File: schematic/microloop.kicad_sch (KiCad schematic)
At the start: 28 parts, among them J1 AudioJack3, J2 AudioJack3, SW1 RotaryEncoder_Switch, SW2 RotaryEncoder_Switch, SW3 RotaryEncoder_Switch, SW4 RotaryEncoder_Switch, SW5 SW_Push, SW6 SW_Push, SW7 SW_Push, SW8 SW_Push, U1 Teensy4.1, U2 Teensy4.0_AudioShield_REVD, U3 Adafruit MIDI Featherwing, U4 Adafruit NeoKey 1x4, U5 MCP23017_SO, U6 128×64 OLED

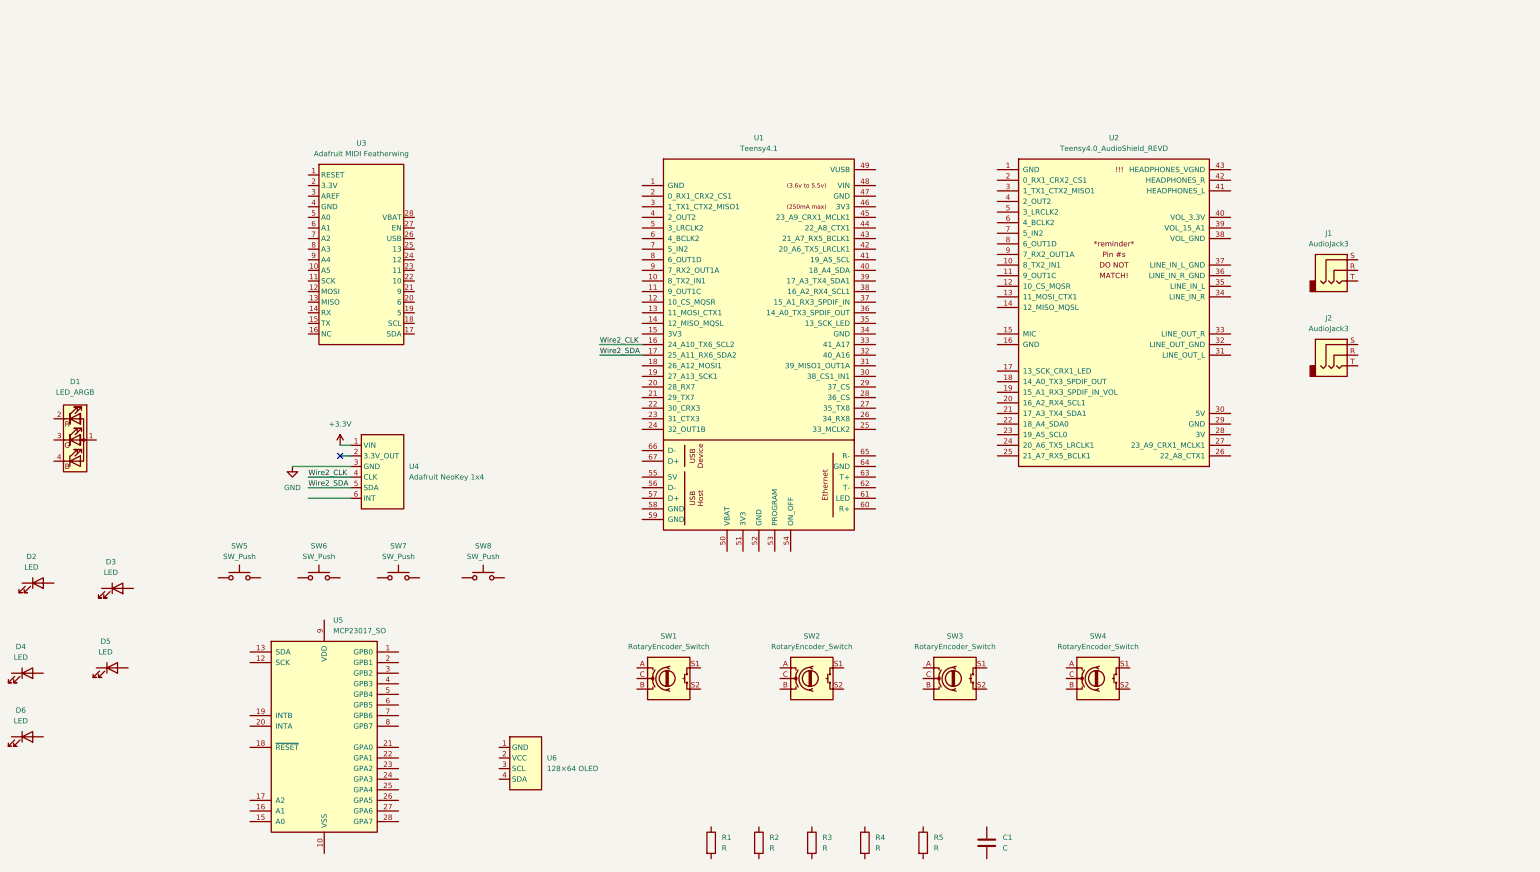
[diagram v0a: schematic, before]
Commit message: updated schematic
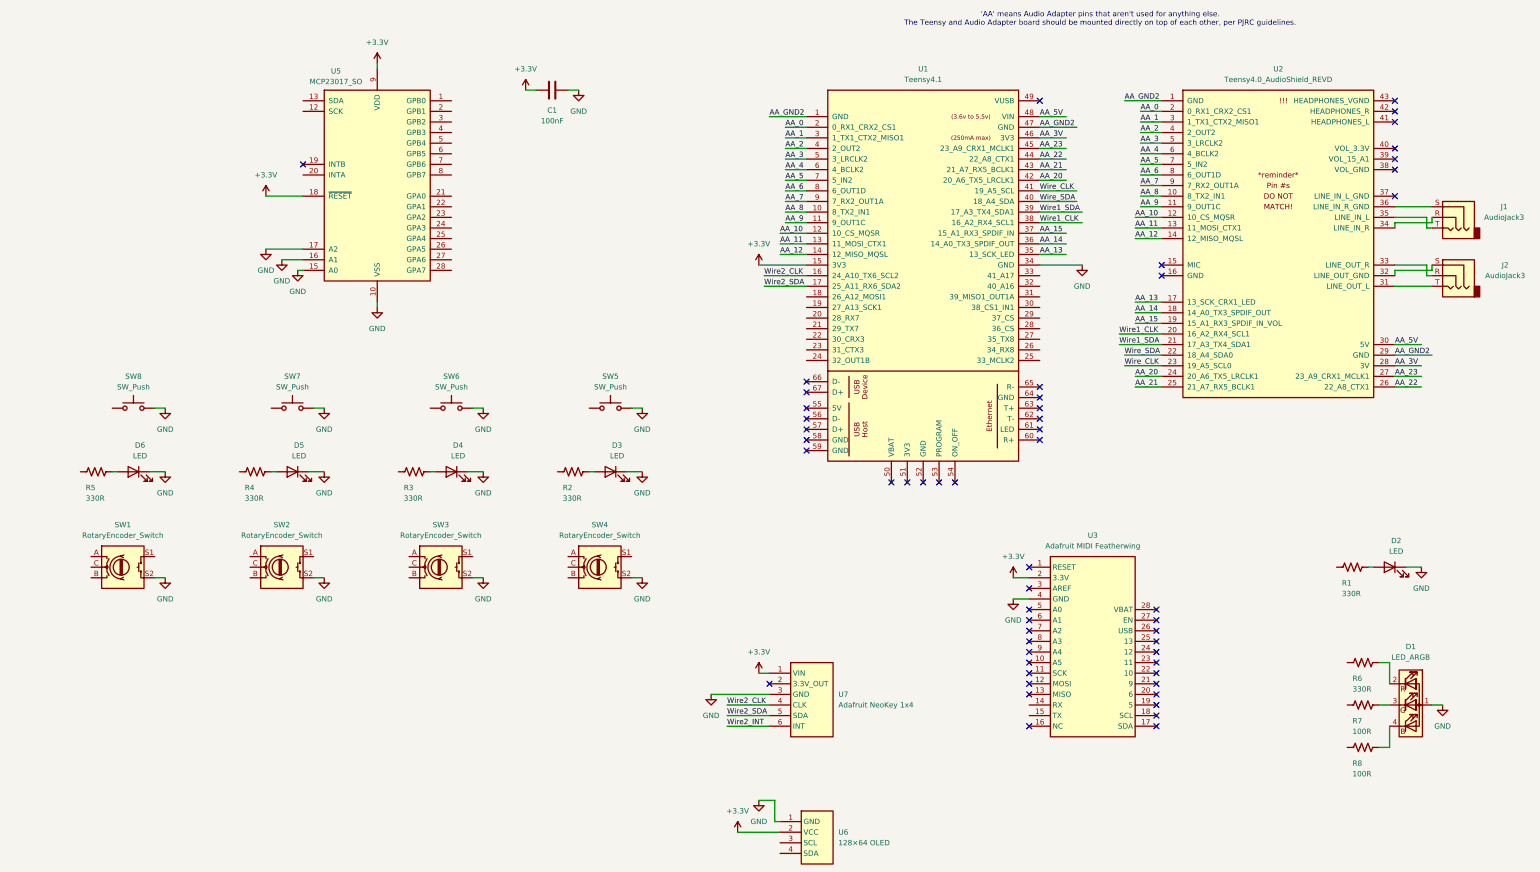
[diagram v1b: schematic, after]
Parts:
- removed R1, R2, R3, R4, R5: R, symbol Device:R
- removed U4: Adafruit NeoKey 1x4, symbol new:neokey
- added R1, R2, R3, R4, R5, R6: 330R, symbol Device:R_US
- added R7, R8: 100R, symbol Device:R_US
- added U7: Adafruit NeoKey 1x4, symbol new:neokey
- C1: value C -> 100nF
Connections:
- net +3.3V: now also C1.1, U1.15 (3V3), U3.2 (3.3V), U5.18 (~{RESET}), U5.9 (VDD), U6.2 (VCC), U7.1 (VIN)
- net GND: now also C1.2, D1.1 (A), D2.1 (K), D3.1 (K), D4.1 (K), D5.1 (K), D6.1 (K), SW1.S2, SW2.S2, SW3.S2, SW4.S2, SW5.1, SW6.1, SW7.1, SW8.1, U1.34 (GND), U3.4 (GND), U5.10 (VSS), U5.15 (A0), U5.16 (A1), U5.17 (A2), U6.1 (GND), U7.3 (GND)
- net Wire2_CLK: now also U7.4 (CLK)
- net Wire2_SDA: now also U7.5 (SDA)
- net at D3.2 (A): now also R2.1
- net at D2.2 (A): now also R1.1
- net AA_GND2: now reaches U1.1 (GND)
- net AA_GND2: now also U1.47 (GND), U2.1 (GND), U2.29 (GND)
- net AA_8: now reaches U1.10 (8_TX2_IN1)
- net AA_8: now also U2.10 (8_TX2_IN1)
- net AA_9: now reaches U1.11 (9_OUT1C)
- net AA_9: now also U2.11 (9_OUT1C)
- net AA_10: now reaches U1.12 (10_CS_MQSR)
- net AA_10: now also U2.12 (10_CS_MQSR)
- net AA_11: now reaches U1.13 (11_MOSI_CTX1)
- net AA_11: now also U2.13 (11_MOSI_CTX1)
- net AA_12: now reaches U1.14 (12_MISO_MQSL)
- net AA_12: now also U2.14 (12_MISO_MQSL)
- net AA_0: now reaches U1.2 (0_RX1_CRX2_CS1)
- net AA_0: now also U2.2 (0_RX1_CRX2_CS1)
- net AA_1: now reaches U1.3 (1_TX1_CTX2_MISO1)
- net AA_1: now also U2.3 (1_TX1_CTX2_MISO1)
- net AA_13: now reaches U1.35 (13_SCK_LED)
- net AA_13: now also U2.17 (13_SCK_CRX1_LED)
- net AA_14: now reaches U1.36 (14_A0_TX3_SPDIF_OUT)
- net AA_14: now also U2.18 (14_A0_TX3_SPDIF_OUT)
- net AA_15: now reaches U1.37 (15_A1_RX3_SPDIF_IN)
- net AA_15: now also U2.19 (15_A1_RX3_SPDIF_IN_VOL)
- net Wire1_CLK: now reaches U1.38 (16_A2_RX4_SCL1)
- net Wire1_CLK: now also U2.20 (16_A2_RX4_SCL1)
- net Wire1_SDA: now reaches U1.39 (17_A3_TX4_SDA1)
- net Wire1_SDA: now also U2.21 (17_A3_TX4_SDA1)
- net AA_2: now reaches U1.4 (2_OUT2)
- net AA_2: now also U2.4 (2_OUT2)
- net Wire_SDA: now reaches U1.40 (18_A4_SDA)
- net Wire_SDA: now also U2.22 (18_A4_SDA0)
- net Wire_CLK: now reaches U1.41 (19_A5_SCL)
- net Wire_CLK: now also U2.23 (19_A5_SCL0)
- net AA_20: now reaches U1.42 (20_A6_TX5_LRCLK1)
- net AA_20: now also U2.24 (20_A6_TX5_LRCLK1)
- net AA_21: now reaches U1.43 (21_A7_RX5_BCLK1)
- net AA_21: now also U2.25 (21_A7_RX5_BCLK1)
- net AA_22: now reaches U1.44 (22_A8_CTX1)
- net AA_22: now also U2.26 (22_A8_CTX1)
- net AA_23: now reaches U1.45 (23_A9_CRX1_MCLK1)
- net AA_23: now also U2.27 (23_A9_CRX1_MCLK1)
- net AA_3V: now reaches U1.46 (3V3)
- net AA_3V: now also U2.28 (3V)
- net AA_5V: now reaches U1.48 (VIN)
- net AA_5V: now also U2.30 (5V)
- net AA_3: now reaches U1.5 (3_LRCLK2)
- net AA_3: now also U2.5 (3_LRCLK2)
- net AA_4: now reaches U1.6 (4_BCLK2)
- net AA_4: now also U2.6 (4_BCLK2)
- net AA_5: now reaches U1.7 (5_IN2)
- net AA_5: now also U2.7 (5_IN2)
- net AA_6: now reaches U1.8 (6_OUT1D)
- net AA_6: now also U2.8 (6_OUT1D)
- net AA_7: now reaches U1.9 (7_RX2_OUT1A)
- net AA_7: now also U2.9 (7_RX2_OUT1A)
- net at J1.R: now also U2.34 (LINE_IN_R)
- net at J1.S: now also U2.36 (LINE_IN_R_GND)
- net at J1.T: now also U2.35 (LINE_IN_L)
- net at U2.31 (LINE_OUT_L): now also J2.T
- net at U2.32 (LINE_OUT_GND): now also J2.S
- net at U2.33 (LINE_OUT_R): now also J2.R
- net at D5.2 (A): now also R4.1
- net at D4.2 (A): now also R3.1
- net at D6.2 (A): now also R5.1
- net at D1.2 (RK): now also R6.1
- net at D1.3 (GK): now also R7.1
- net at D1.4 (BK): now also R8.1
- new net Wire2_INT: U7.6 (INT)
- no-connect marks 1 -> 54
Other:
- note added: "'AA' means Audio Adapter pins that aren't used for anything else. The Teensy and Audio Adapter board should be mounted directly on top of each other, per PJRC guidelines."
- moved on the sheet: C1, D1, D2, J1, J2, SW1, SW2, SW3, SW4, SW5, SW6, SW7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
